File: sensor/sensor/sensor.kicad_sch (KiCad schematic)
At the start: 13 parts, among them J1 RJ12_Shielded, J2 Conn_01x04, J3 Conn_01x06, U1 PCA9615DP, U2 LTC4316xDD, U3 APDS-9960, U4 TPS76301

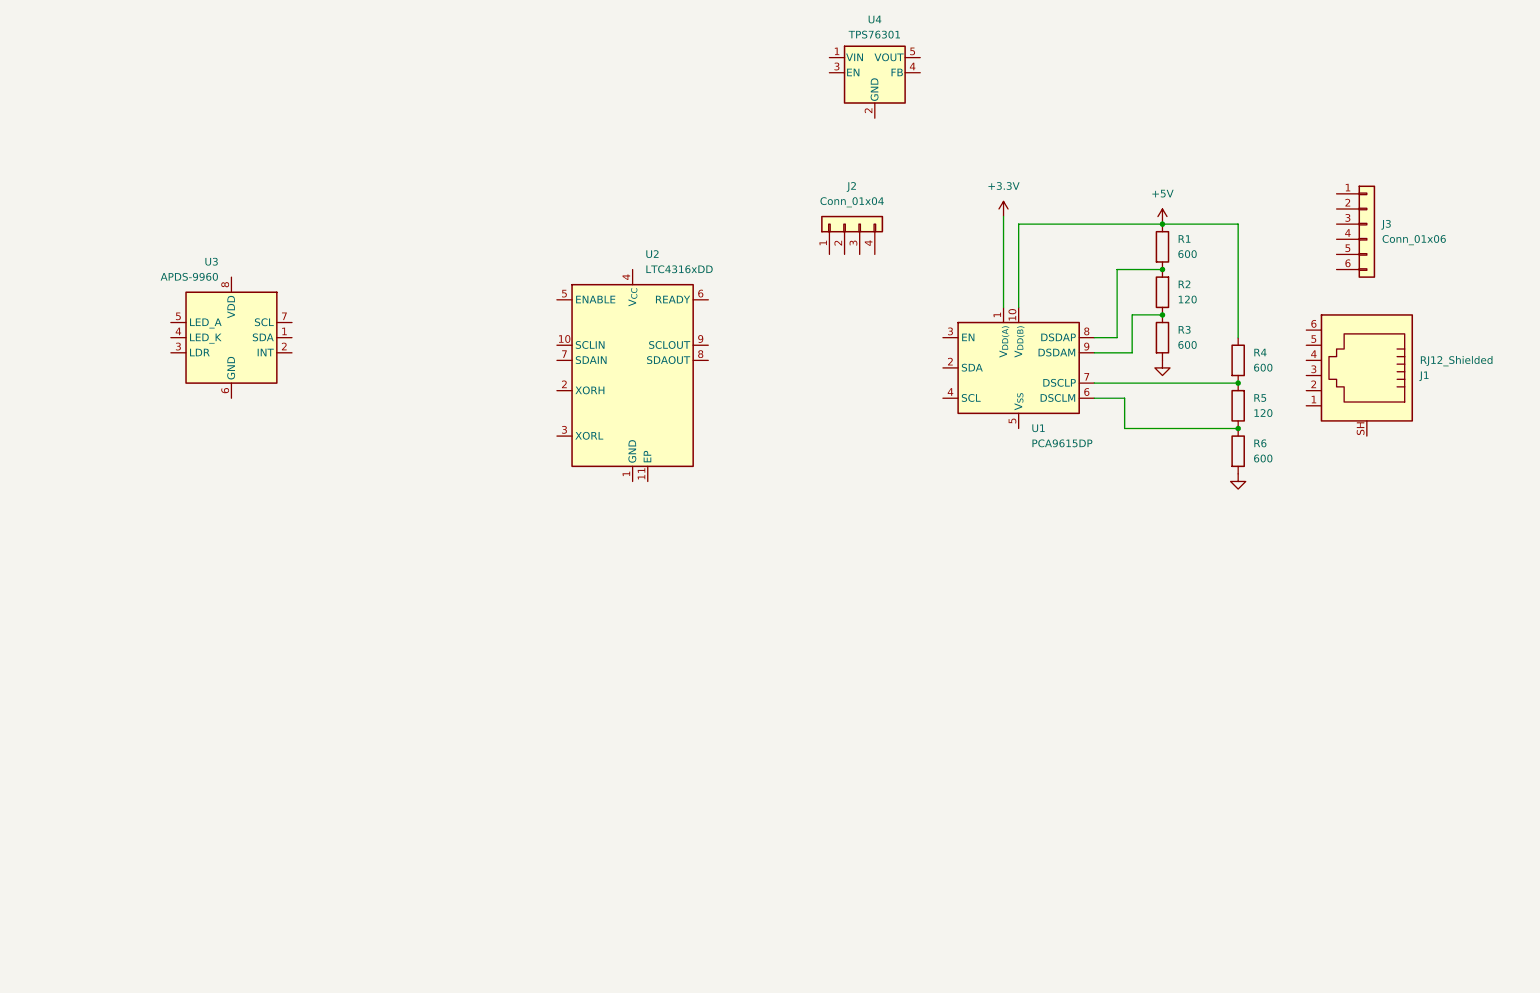
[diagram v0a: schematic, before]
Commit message: update sensor
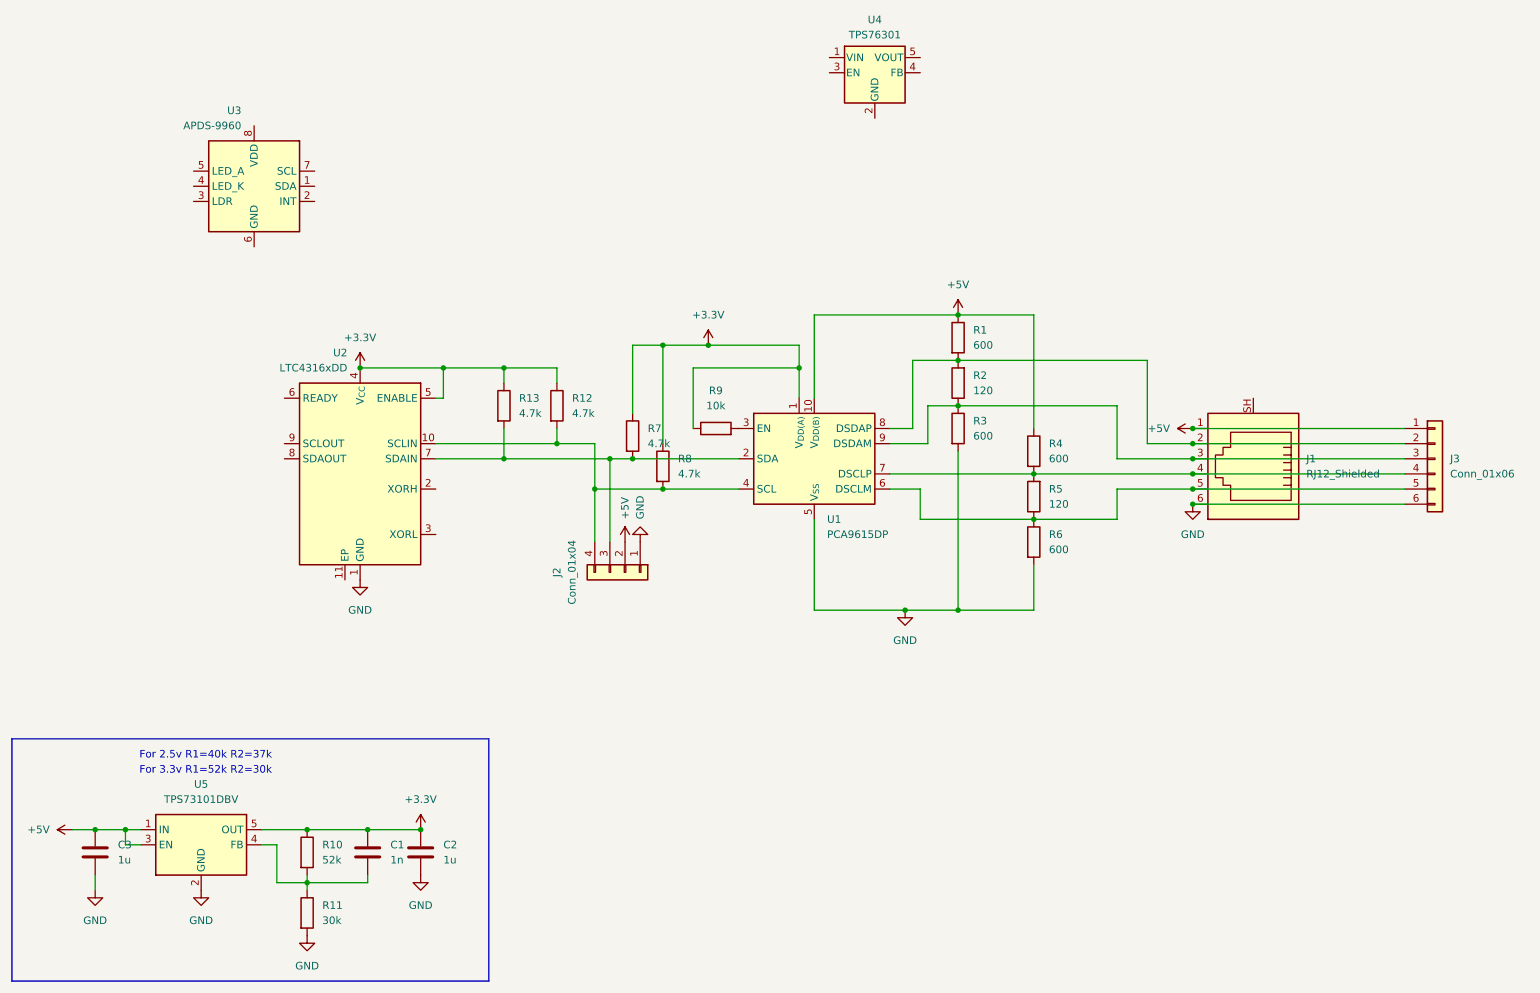
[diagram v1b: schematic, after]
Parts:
- added C1: 1n, symbol Device:C
- added C2, C3: 1u, symbol Device:C
- added R10: 52k, symbol Device:R
- added R11: 30k, symbol Device:R
- added R12, R13, R7, R8: 4.7k, symbol Device:R
- added R9: 10k, symbol Device:R
- added U5: TPS73101DBV, Package_TO_SOT_SMD:SOT-23-5, symbol Regulator_Linear:TPS73101DBV
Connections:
- net +3.3V: now also U2.4 (V_{CC}), U2.5 (ENABLE), C1.1, C2.1, R10.1, R12.1, R13.1, R7.1, R8.1, R9.1, U5.5 (OUT)
- net +5V: now also J1.1, J2.2 (Pin_2), J3.1 (Pin_1), C3.1, U5.1 (IN), U5.3 (EN)
- net GND: now also J1.6, J2.1 (Pin_1), J3.6 (Pin_6), U1.5 (V_{SS}), U2.1 (GND), C2.2, C3.2, R11.2, U5.2 (GND)
- net at U2.10 (SCLIN): now also J2.4 (Pin_4), U1.4 (SCL), R12.2, R8.2
- net at U2.7 (SDAIN): now also J2.3 (Pin_3), U1.2 (SDA), R13.2, R7.2
- net at R1.2, R2.2, U1.8 (DSDAP): now also J1.2, J3.2 (Pin_2)
- net at J3.3 (Pin_3): now also J1.3, R2.1, R3.1, U1.9 (DSDAM)
- net at J3.4 (Pin_4): now also J1.4, R4.2, R5.2, U1.7 (DSCLP)
- net at J3.5 (Pin_5): now also J1.5, R5.1, R6.1, U1.6 (DSCLM)
- net at U1.3 (EN): now also R9.2
- new net: C1.2, R10.2, R11.1, U5.4 (FB)
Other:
- note added: "For 2.5v R1=40k R2=37k"
- note added: "For 3.3v R1=52k R2=30k"
- moved on the sheet: J1, J2, J3, R1, R2, R3, R4, R5, R6, U1, U2, U3
